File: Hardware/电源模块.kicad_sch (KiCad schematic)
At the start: 33 parts, among them J1 Barrel_Jack_Switch, U5 AMS1117-1.8, U6 AMS1117-2.5, U7 AMS1117-3.3, U8 MP2315GJ

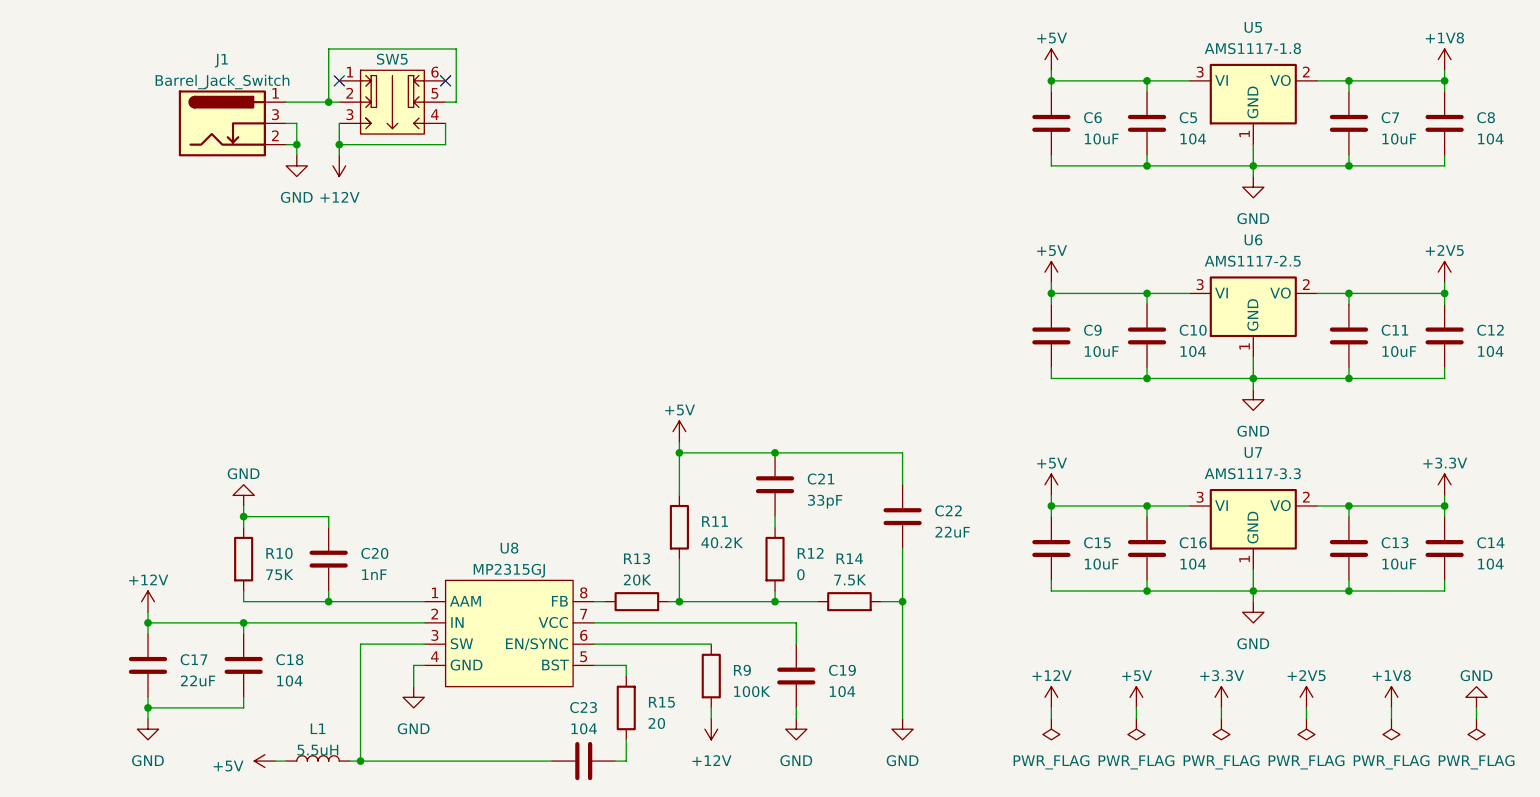
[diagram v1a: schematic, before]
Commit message: 2023/3/29
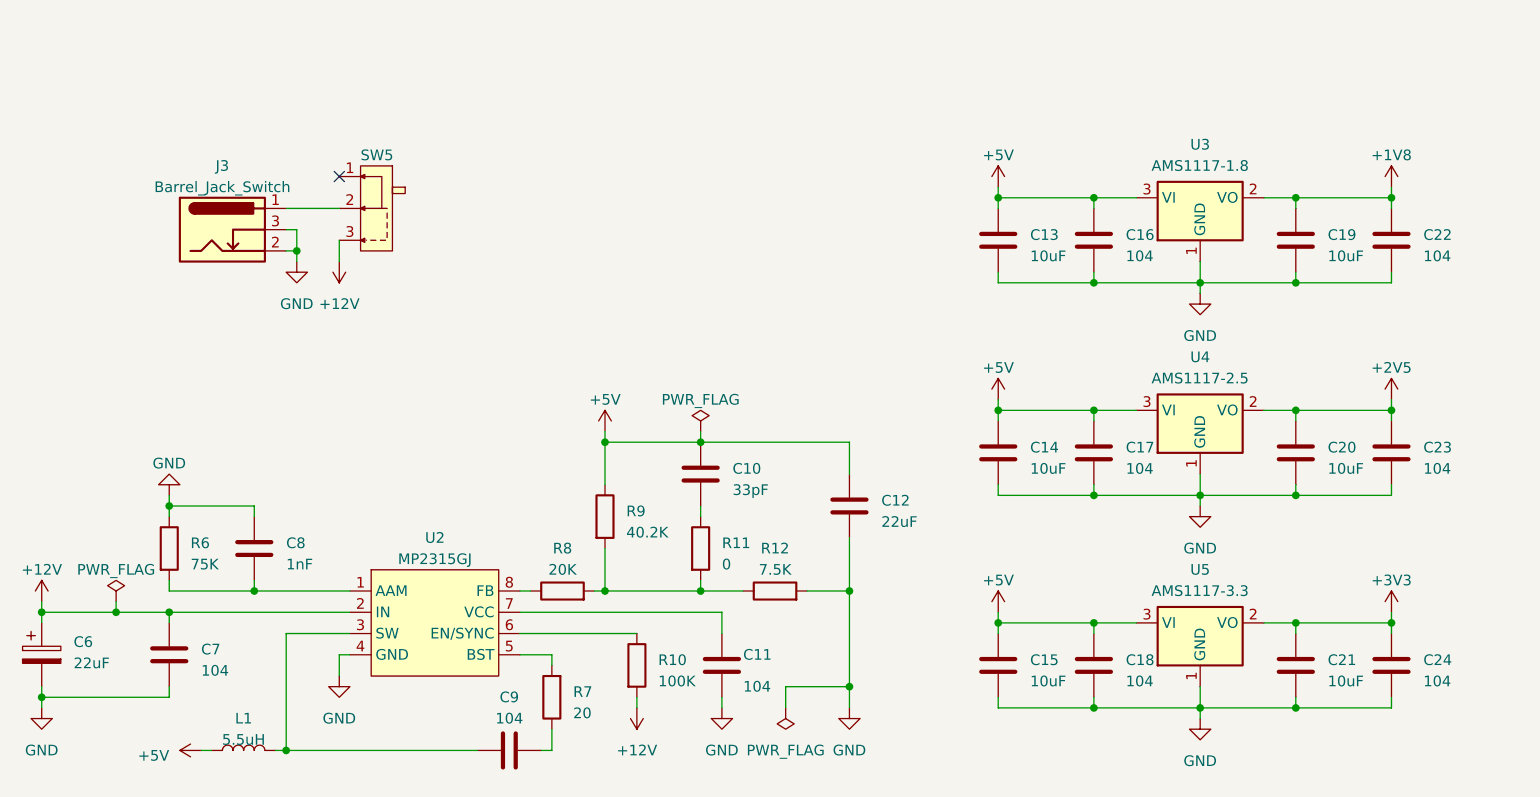
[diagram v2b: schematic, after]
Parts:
- removed C17: 22uF, symbol Device:C
- removed SW5: ~, Switching_Devices:Self_Locking_Switch_5.8_5.8, symbol Switching_Devices:Self_Locking_Switch
- added C6: 22uF, Capacitor_SMD:CP_Elec_4x5.4, symbol Device:C_Polarized
- added SW5: ~, symbol Library:SW
- C10: renamed from C21; footprint (none) -> Capacitor_SMD:C_0402_1005Metric
- C11: renamed from C19; footprint (none) -> Capacitor_SMD:C_0402_1005Metric
- C12: renamed from C22; footprint (none) -> Capacitor_SMD:C_1206_3216Metric
- C13: renamed from C6; footprint (none) -> Capacitor_SMD:C_0603_1608Metric
- C14: renamed from C9; footprint (none) -> Capacitor_SMD:C_0603_1608Metric
- C15: footprint (none) -> Capacitor_SMD:C_0603_1608Metric
- C16: renamed from C5; footprint (none) -> Capacitor_SMD:C_0402_1005Metric
- C17: renamed from C10; footprint (none) -> Capacitor_SMD:C_0402_1005Metric
- C18: renamed from C16; footprint (none) -> Capacitor_SMD:C_0402_1005Metric
- C19: renamed from C7; footprint (none) -> Capacitor_SMD:C_0603_1608Metric
- C20: renamed from C11; footprint (none) -> Capacitor_SMD:C_0603_1608Metric
- C21: renamed from C13; footprint (none) -> Capacitor_SMD:C_0603_1608Metric
- C22: renamed from C8; footprint (none) -> Capacitor_SMD:C_0402_1005Metric
- C23: renamed from C12; footprint (none) -> Capacitor_SMD:C_0402_1005Metric
- C24: renamed from C14; footprint (none) -> Capacitor_SMD:C_0402_1005Metric
- C7: renamed from C18; footprint (none) -> Capacitor_SMD:C_0402_1005Metric
- C8: renamed from C20; footprint (none) -> Capacitor_SMD:C_0402_1005Metric
- C9: renamed from C23; footprint (none) -> Capacitor_SMD:C_0402_1005Metric
- J3: renamed from J1; footprint (none) -> Connector_BarrelJack:BarrelJack_CLIFF_FC681465S_SMT_Horizontal
- L1: footprint (none) -> Inductor_SMD:L_2512_6332Metric_Pad1.52x3.35mm_HandSolder
- R10: renamed from R9; footprint (none) -> Resistor_SMD:R_0402_1005Metric
- R11: renamed from R12; footprint (none) -> Resistor_SMD:R_0402_1005Metric
- R12: renamed from R14; footprint (none) -> Resistor_SMD:R_0402_1005Metric
- R6: renamed from R10; footprint (none) -> Resistor_SMD:R_0402_1005Metric
- R7: renamed from R15; footprint (none) -> Resistor_SMD:R_0402_1005Metric
- R8: renamed from R13; footprint (none) -> Resistor_SMD:R_0402_1005Metric
- R9: renamed from R11; footprint (none) -> Resistor_SMD:R_0402_1005Metric
- renumbered U8 to U2, U5 to U3, U6 to U4, U7 to U5
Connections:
- net +12V: now also C6.1, SW5.3
- net GND: now also C6.2
- net at J3.1: now also SW5.2
- net +3.3V renamed +3V3
- no-connect marks 2 -> 1
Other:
- moved on the sheet: C10, C11, C12, C13, C14, C15, C16, C17, C18, C19, C20, C21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
